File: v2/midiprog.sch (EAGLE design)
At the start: 56 parts, among them IC1 PIC18F4550_40, IC2 TPIC6B596N, IC3 78L05Z, IC4 TPIC6B596N, Q1 8MHz, Q2 2N2222A, Q3 2N2222A, Q4 2N2222A

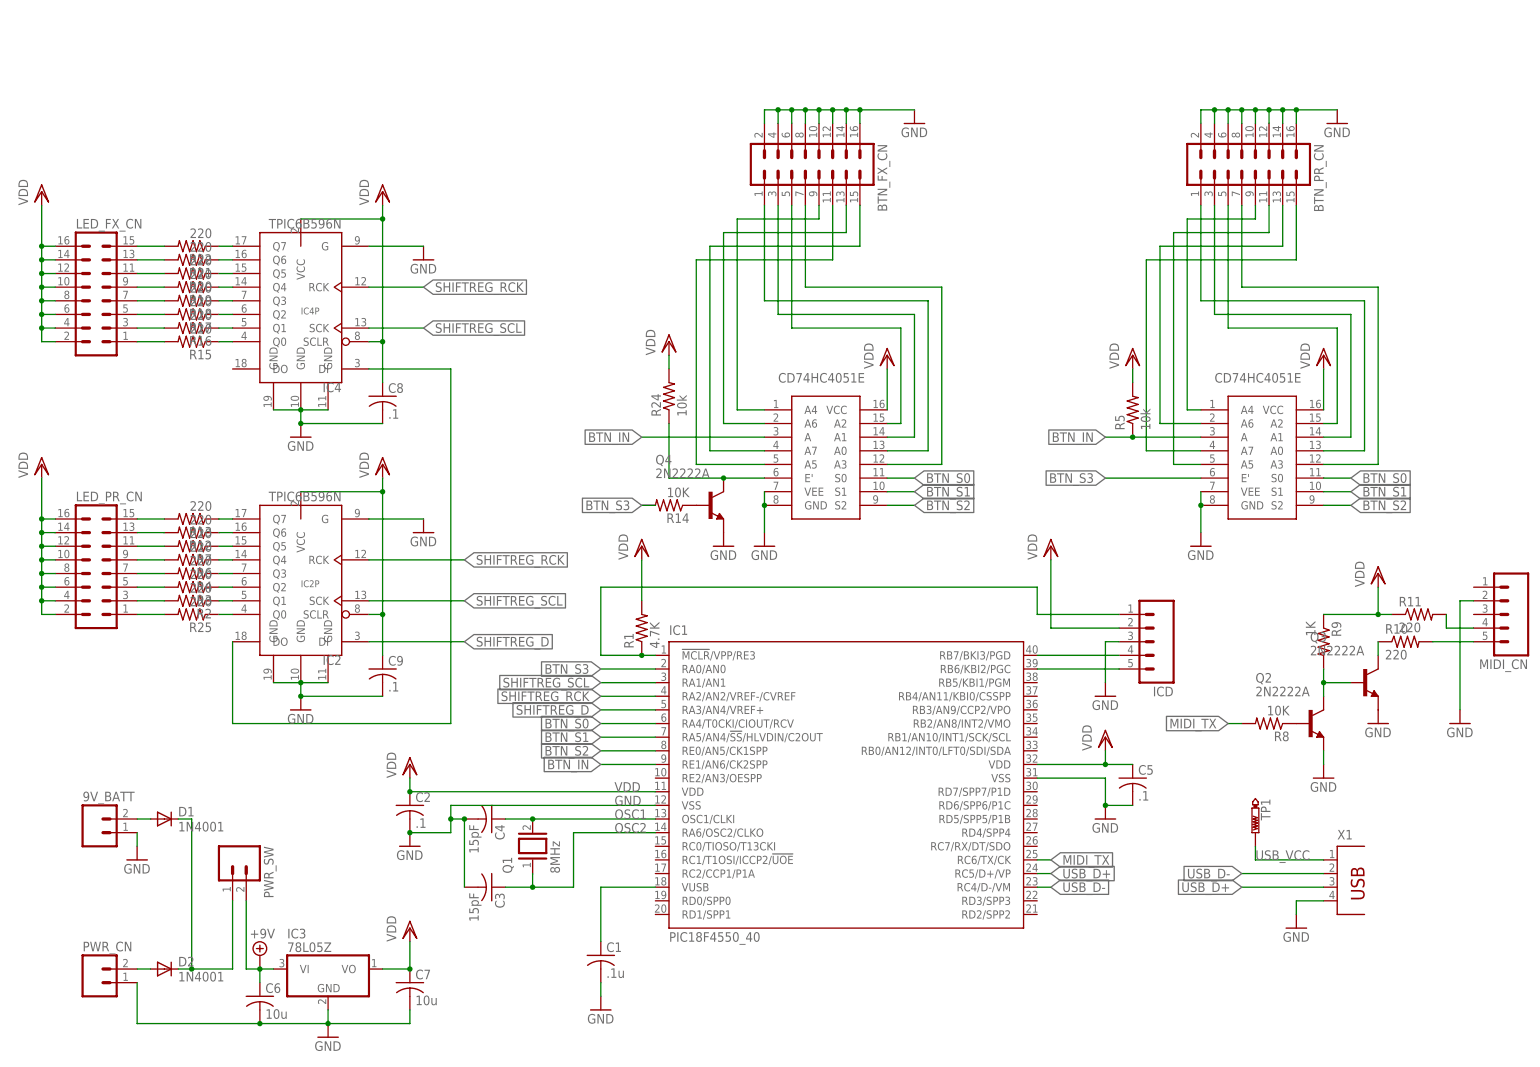
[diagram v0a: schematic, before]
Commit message: Decent layout; not great.
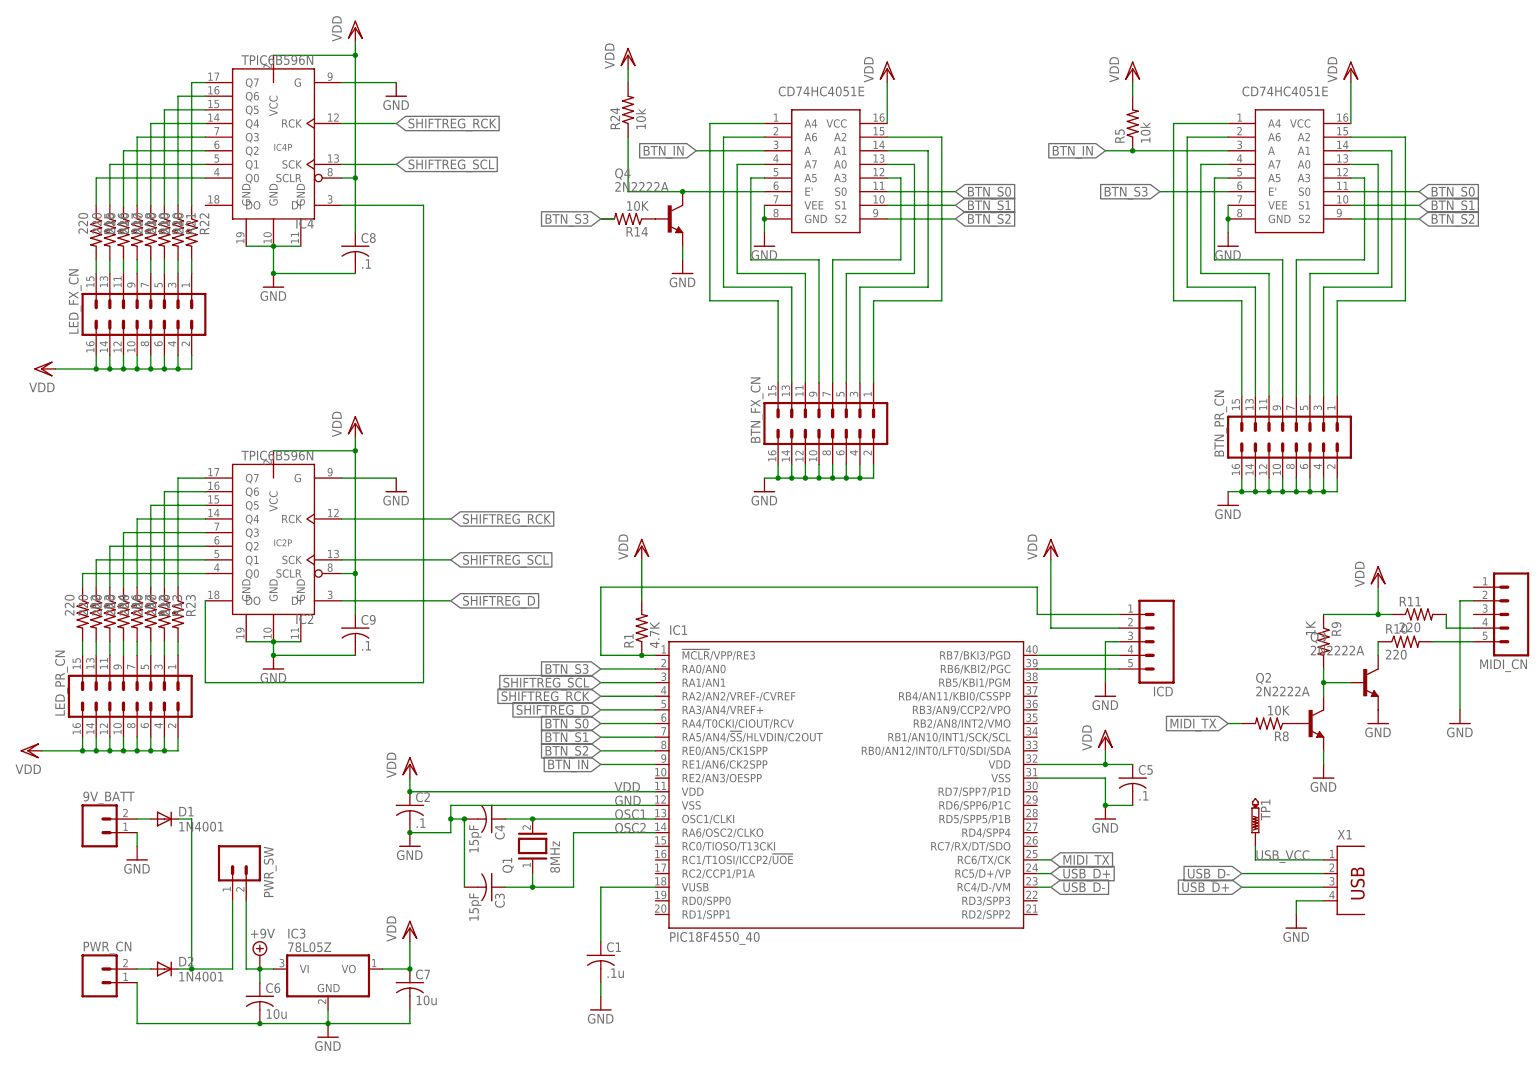
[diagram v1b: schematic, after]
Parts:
- removed R25: 220, rcl:R-US_0207/10
- added R23: 220, rcl:R-US_0207/10
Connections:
- net BFX2 renamed N$63
- net BFX4 renamed N$61
- net BFX7 renamed N$49
- net BPR2 renamed N$57
- net BPR4 renamed N$55
- net BPR7 renamed N$51
- removed net BFX1: BTN_FX_CN.1, U$2.A0
- removed net BFX3: BTN_FX_CN.5, U$2.A2
- removed net BFX5: BTN_FX_CN.9, U$2.A4
- removed net BFX6: BTN_FX_CN.11, U$2.A5
- removed net BFX8: BTN_FX_CN.15, U$2.A7
- removed net BPR1: BTN_PR_CN.1, U$1.A0
- removed net BPR3: BTN_PR_CN.5, U$1.A2
- removed net BPR5: BTN_PR_CN.9, U$1.A4
- removed net BPR6: BTN_PR_CN.11, U$1.A5
- removed net BPR8: BTN_PR_CN.15, U$1.A7
- removed net N$19 (its old number): LED_FX_CN.9, R19.2
- removed net N$20 (its old number): LED_FX_CN.7, R18.2
- removed net N$21 (its old number): LED_FX_CN.5, R17.2
- removed net N$22 (its old number): LED_FX_CN.3, R16.2
- removed net N$23 (its old number): LED_FX_CN.1, R15.2
- new net N$10: LED_FX_CN.11, R17.2
- new net N$13: LED_FX_CN.5, R20.2
- new net N$14: LED_FX_CN.3, R21.2
- new net N$15: LED_FX_CN.1, R22.2
- new net N$3: LED_FX_CN.13, R16.2
- new net N$46: BTN_FX_CN.9, U$2.A5
- new net N$47: BTN_PR_CN.9, U$1.A5
- new net N$48: BTN_FX_CN.11, U$2.A7
- new net N$50: BTN_PR_CN.11, U$1.A7
- new net N$52: BTN_PR_CN.15, U$1.A4
- new net N$56: BTN_PR_CN.5, U$1.A0
- new net N$58: BTN_PR_CN.1, U$1.A2
- new net N$60: BTN_FX_CN.15, U$2.A4
- new net N$62: BTN_FX_CN.5, U$2.A0
- new net N$64: BTN_FX_CN.1, U$2.A2
- net N$11: now also LED_FX_CN.9, R18.2; no longer LED_FX_CN.13, R21.2
- net N$12: now also LED_FX_CN.7, R19.2; no longer LED_FX_CN.11, R20.2
- net N$2: now also R15.2; no longer R22.2
- net N$24: now also R3.2; no longer R12.2
- net N$27: now also R4.2; no longer R7.2
- net N$30: now also R7.2; no longer R4.2
- net N$32: now also R12.2; no longer R3.2
- net N$36: now also R13.2; no longer R2.2
- net N$37: now also R23.2; no longer R25.2
- net N$38: now also IC2G$1.Q0, R2.1; no longer IC2G$1.Q7, R13.1
- net N$39: now also IC2G$1.Q1, R3.1; no longer IC2G$1.Q6, R12.1
- net N$40: now also IC2G$1.Q2, R4.1; no longer IC2G$1.Q5, R7.1
- net N$41: now also IC2G$1.Q3; no longer IC2G$1.Q4
- net N$42: now also IC2G$1.Q4, R7.1; no longer IC2G$1.Q3, R4.1
- net N$43: now also IC2G$1.Q5, R12.1; no longer IC2G$1.Q2, R3.1
- net N$44: now also IC2G$1.Q6, R13.1; no longer IC2G$1.Q1, R2.1
- net N$45: now also IC2G$1.Q7, R23.1; no longer IC2G$1.Q0, R25.1
- net N$6: now also R2.2; no longer R13.2
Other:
- moved on the sheet: BTN_FX_CN, BTN_PR_CN, C8, C9, IC2, IC2P, IC4, IC4P, LED_FX_CN, LED_PR_CN, Q4, R12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
